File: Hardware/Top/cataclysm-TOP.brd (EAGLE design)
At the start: 38 x 38 mm, 58 parts, among them SW3 SWITCH.MOM, SW4 SWITCH.MOM, U1 NRF52832_MODULE_MDBT42, U3 FT231XS, Y1 32.768kHz

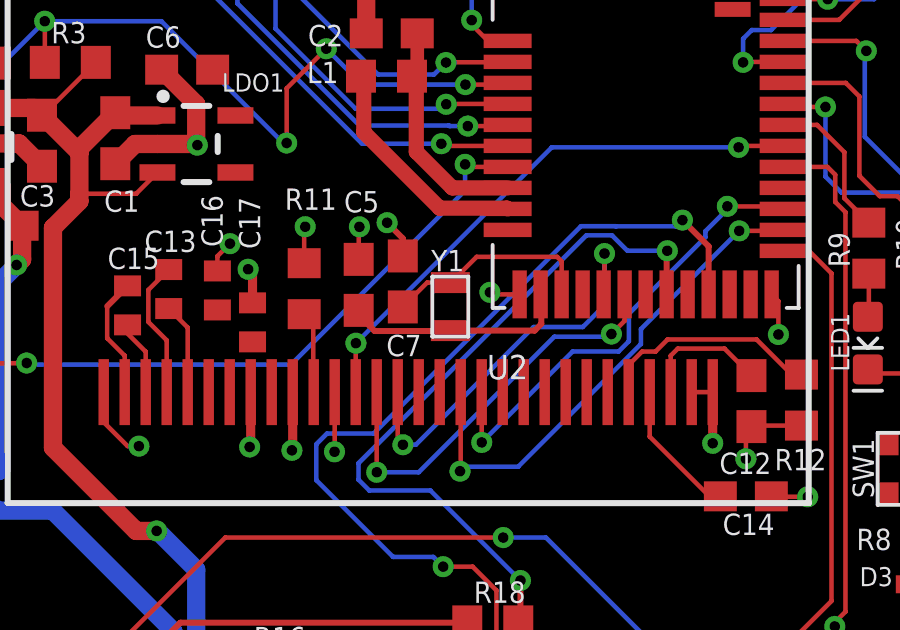
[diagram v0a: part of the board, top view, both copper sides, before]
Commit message: Take 7 Done w/ no airwire
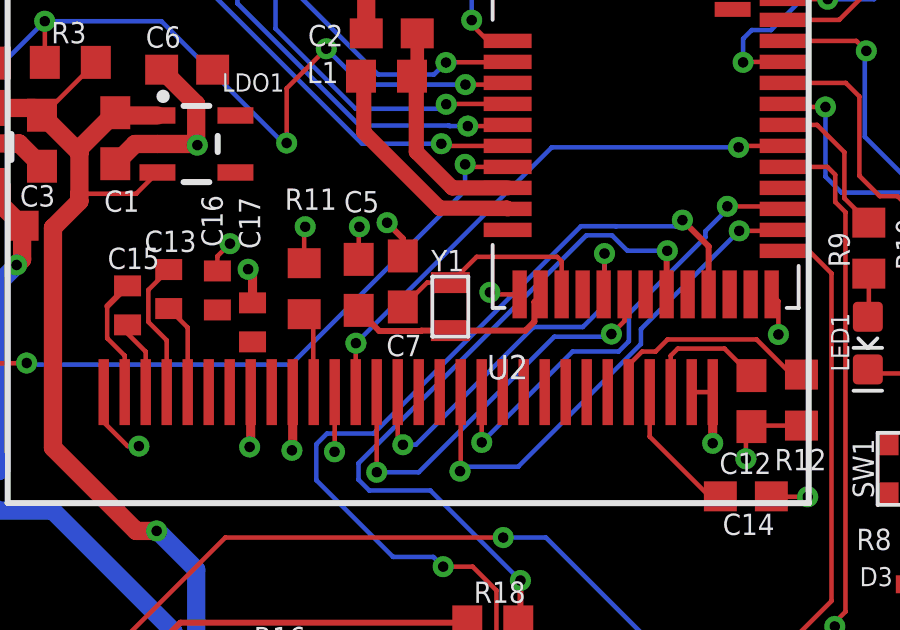
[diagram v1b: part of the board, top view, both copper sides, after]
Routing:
- net N$4: track 8.03 -> 7.44 mm
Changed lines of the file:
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@@
 <contactref element="Y1" pad="P$1"/>
 <contactref element="U1" pad="13"/>
-<wire x1="18.060278125" y1="20.812853125" x2="17.89208125" y2="20.64465625" width="0.1524" layer="1"/>
 <wire x1="15.392403125" y1="21.362296875" x2="15.392403125" y2="21.204815625" width="0.1524" layer="1"/>
-<wire x1="18.279821875" y1="20.52019375" x2="18.44801875" y2="20.688390625" width="0.1524" layer="1"/>
-<wire x1="18.44801875" y1="20.688390625" x2="18.43381875" y2="20.674190625" width="0.2" layer="1"/>
-<wire x1="18.43381875" y1="20.674190625" x2="15.923028125" y2="20.674190625" width="0.2" layer="1"/>
-<wire x1="15.392403125" y1="21.204815625" x2="15.923028125" y2="20.674190625" width="0.2" layer="1"/>
-<wire x1="18.44801875" y1="20.688390625" x2="21.259890625" y2="20.688390625" width="0.2" layer="1"/>
-<wire x1="21.259890625" y1="20.688390625" x2="21.48078125" y2="20.90928125" width="0.2" layer="1"/>
-<wire x1="21.48078125" y1="20.90928125" x2="21.48078125" y2="21.872540625" width="0.2" layer="1"/>
 <wire x1="21.48078125" y1="21.872540625" x2="21.45804375" y2="21.895278125" width="0.2" layer="1"/>
-<wire x1="18.279821875" y1="20.52019375" x2="18.060278125" y2="20.812853125" width="0" layer="19" extent="1-1"/>
+<wire x1="15.392403125" y1="21.362296875" x2="16.080509375" y2="20.674190625" width="0.2" layer="1"/>
+<wire x1="16.080509375" y1="20.674190625" x2="17.467603125" y2="20.674190625" width="0.2" layer="1"/>
+<wire x1="21.250440625" y1="20.990728125" x2="21.250440625" y2="21.6422" width="0.2" layer="1"/>
+<wire x1="21.250440625" y1="21.6422" x2="21.48078125" y2="21.872540625" width="0.2" layer="1"/>
+<wire x1="20.948103125" y1="20.688390625" x2="21.250440625" y2="20.990728125" width="0.2" layer="1"/>
+<wire x1="17.467603125" y1="20.674190625" x2="17.481803125" y2="20.688390625" width="0.2" layer="1"/>
+<wire x1="17.481803125" y1="20.688390625" x2="18.44801875" y2="20.688390625" width="0.2" layer="1"/>
+<wire x1="18.44801875" y1="20.688390625" x2="20.948103125" y2="20.688390625" width="0.2" layer="1"/>
 </signal>
 <signal name="N$6">
